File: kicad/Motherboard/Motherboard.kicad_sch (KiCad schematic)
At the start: 75 parts, among them J1 USB_C_Receptacle_USB2.0, J10 Conn_01x08_Pin, J11 Conn_01x08_Pin, J12 Conn_01x08_Pin, J13 Conn_01x08_Pin, J2 Conn_01x02_Pin, J3 Conn_01x04_Pin, J4 Conn_01x04_Pin, J5 Conn_01x02_Pin, J6 Conn_01x08_Pin, J7 Conn_01x08_Pin, J8 Conn_01x08_Pin, J9 Conn_01x08_Pin, Q1 DMN3404L, SW1 Reset, SW2 Boot, U1 ESP32-S2-SOLO, U2 LD1117S33TR_SOT223, U3 TCA9535RTWR, U4 TCA9535RTWR, U5 TCA9535RTWR, U6 TCA9535RTWR, U7 TMC2209-LA, U8 TMC2209-LA, U9 LM2575-5.0BT

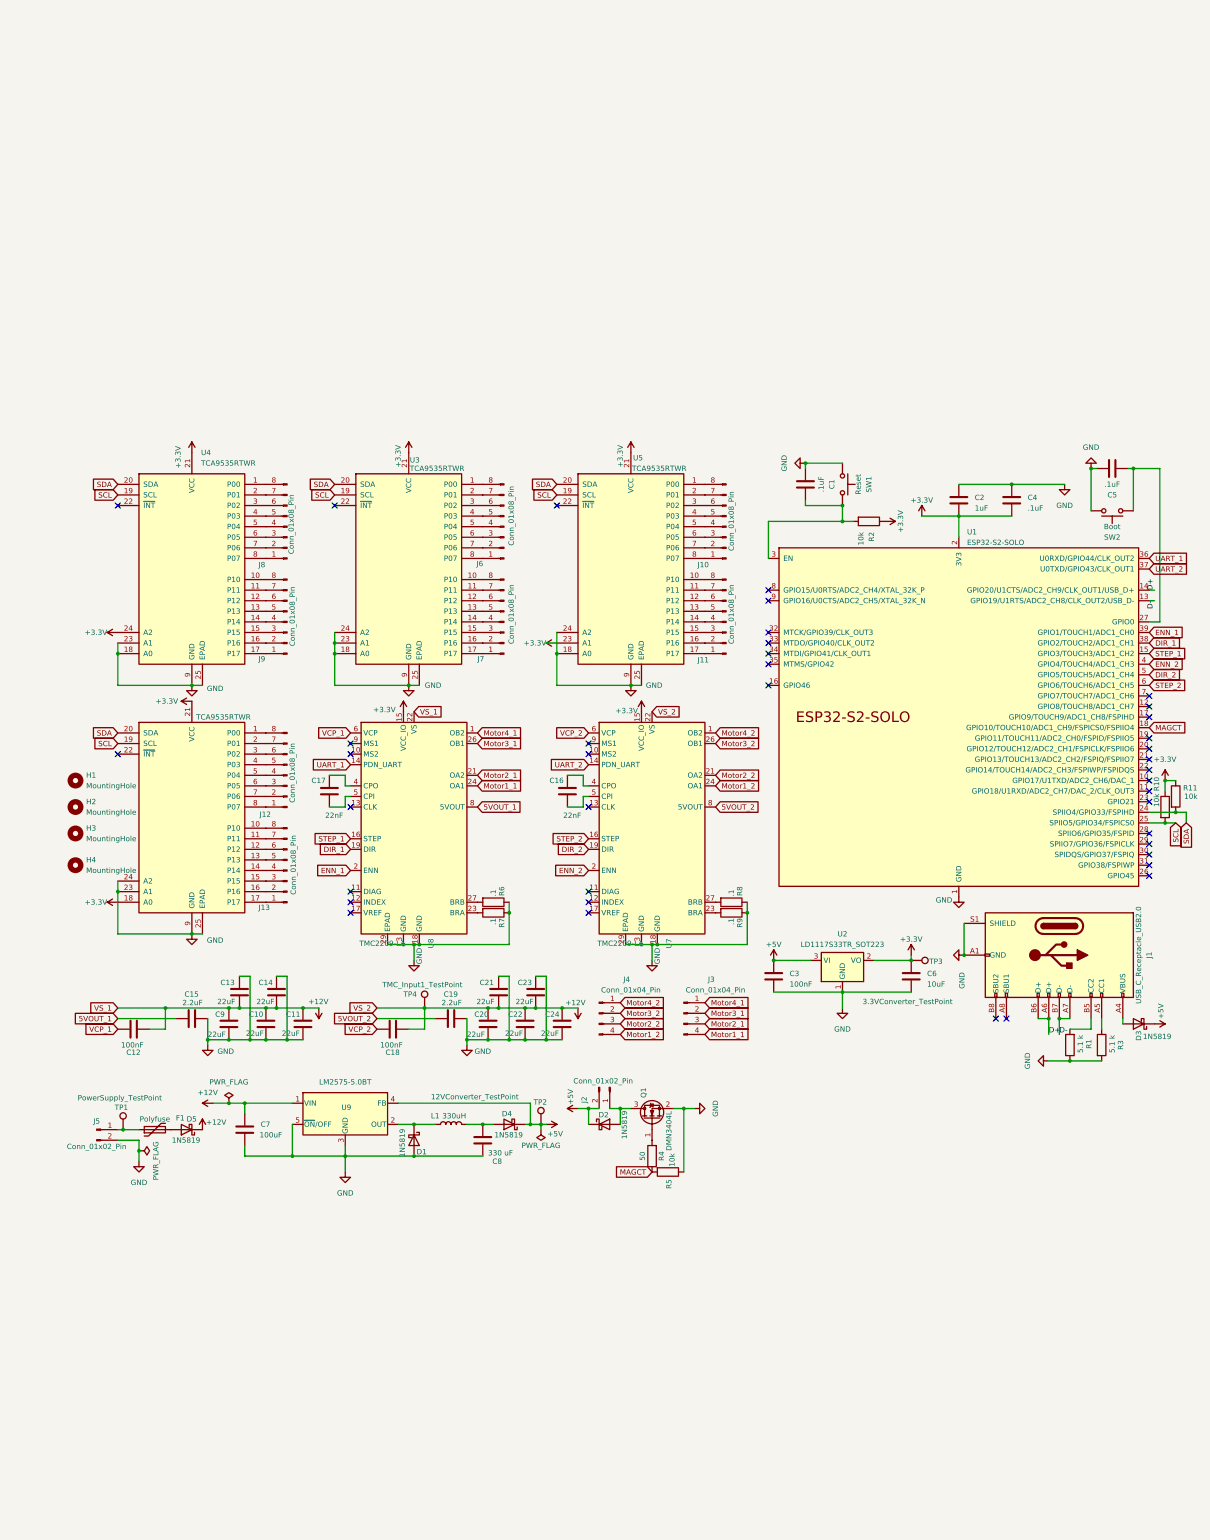
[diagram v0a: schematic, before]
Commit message: added new parts
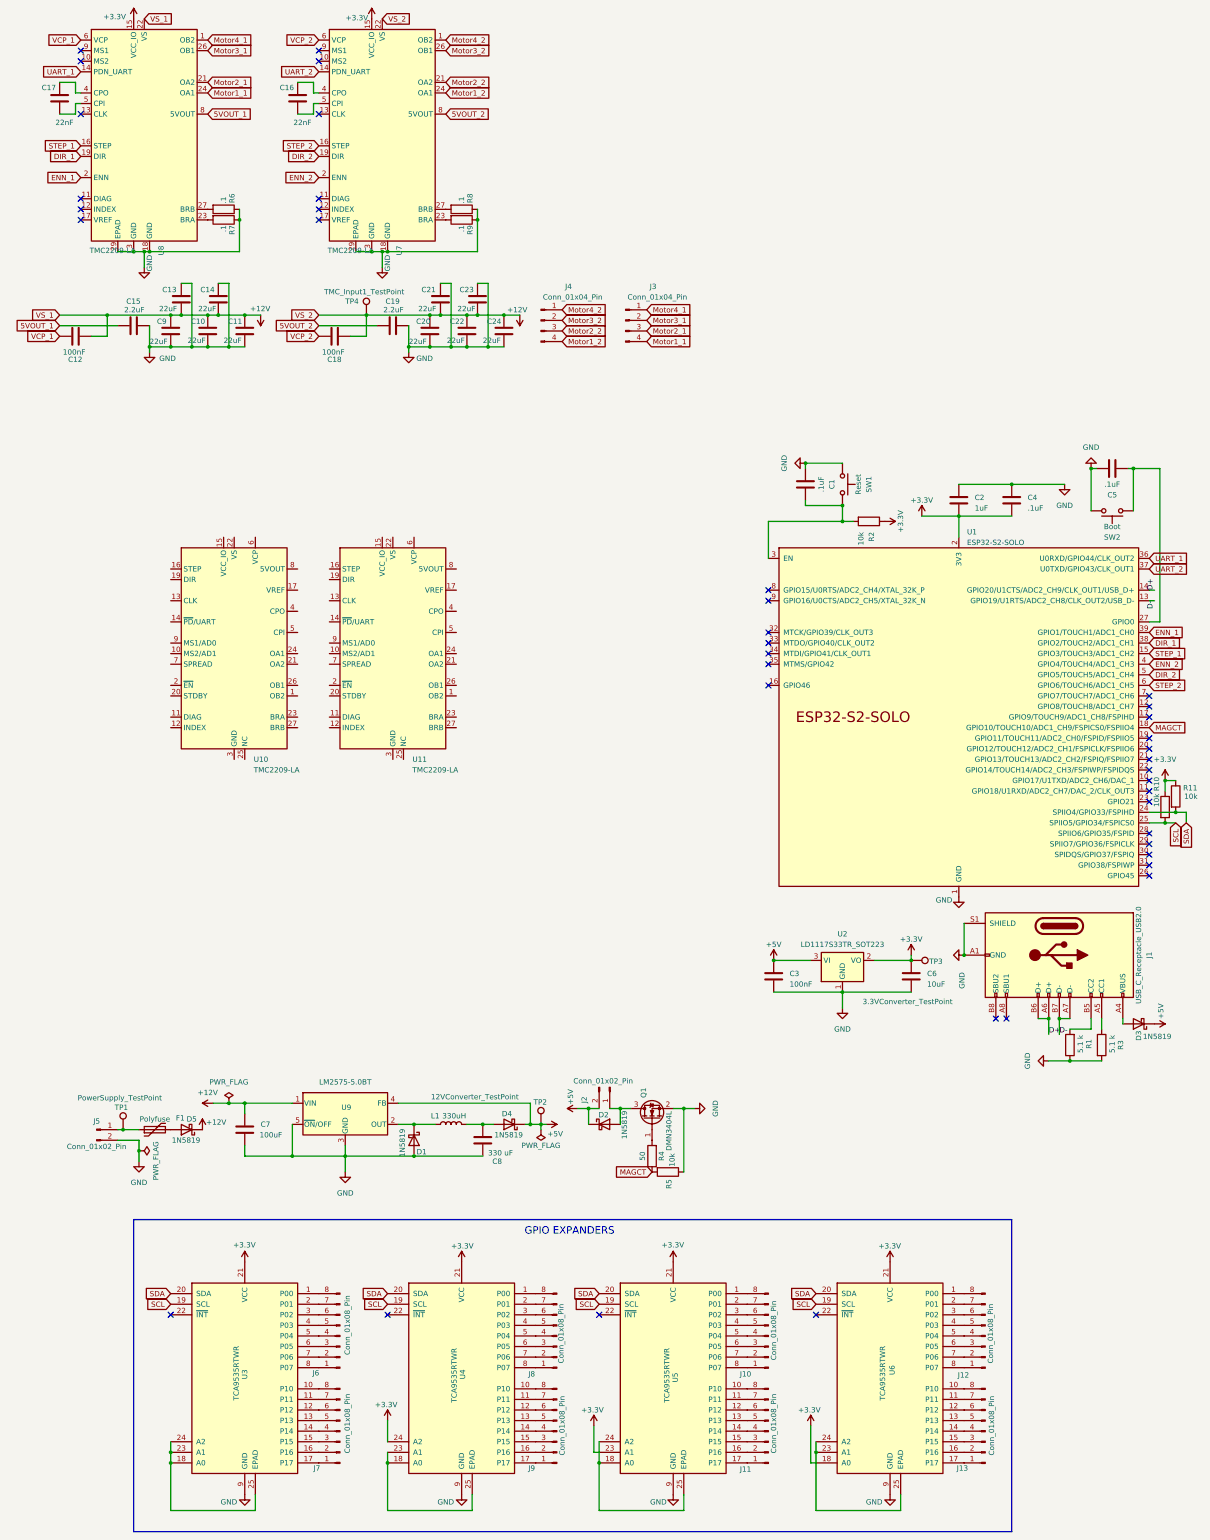
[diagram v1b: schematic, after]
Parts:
- removed H1, H2, H3, H4: MountingHole, symbol Mechanical:MountingHole
- added U10, U11: TMC2209-LA, Package_DFN_QFN:VQFN-28-1EP_5x5mm_P0.5mm_EP3.7x3.7mm_ThermalVias, symbol Driver_Motor:TMC2209-LA
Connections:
- net GND: no longer U3.18 (A0), U3.23 (A1), U3.24 (A2), U3.25 (EPAD), U4.18 (A0), U4.23 (A1), U4.25 (EPAD), U5.18 (A0), U5.24 (A2), U5.25 (EPAD), U6.23 (A1), U6.24 (A2), U6.25 (EPAD)
- new net: U4.18 (A0), U4.23 (A1), U4.25 (EPAD)
- new net: U6.23 (A1), U6.24 (A2), U6.25 (EPAD)
- new net: U5.18 (A0), U5.24 (A2), U5.25 (EPAD)
- new net: U10.18 (GND), U10.29 (GND), U10.3 (GND)
- new net: U10.22 (VS), U10.28 (VS)
- new net: U11.18 (GND), U11.29 (GND), U11.3 (GND)
- new net: U11.22 (VS), U11.28 (VS)
- new net: U3.18 (A0), U3.23 (A1), U3.24 (A2), U3.25 (EPAD)
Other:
- note added: "GPIO EXPANDERS"
- moved on the sheet: C10, C11, C12, C13, C14, C15, C16, C17, C18, C19, C20, C21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
